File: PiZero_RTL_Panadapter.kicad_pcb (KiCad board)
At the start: 4 copper layers, 65 x 30 mm, 196 parts, among them J1 Conn_01x02, J2 JST GH 8 Position, J3 U.FL, J4 U.FL, J5 Conn_01x08, Q1 S8050T, Q2 BFS17, Q3 J310, Q4 BFS17, T1 DXW21BN2511NL, U1 RPM5.0-2.0, U10 SI5351B-B-GM1, U2 AP2114HA-3.3, U4 Raspberry Pi Zero 2W, U5 RTL2832U, U6 M24C02-WMN, U7 FE1.1s, U8 RTL8152B, U9 R820T2, Y1 25MHz

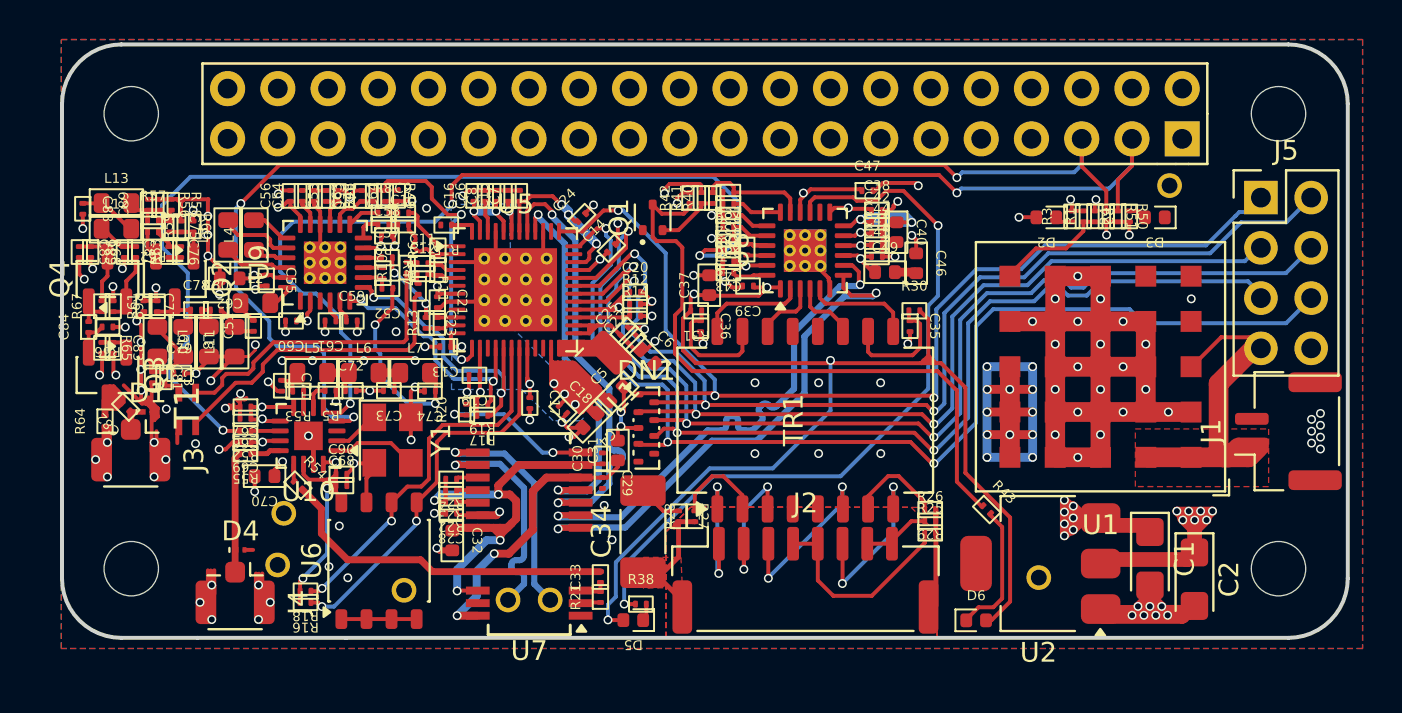
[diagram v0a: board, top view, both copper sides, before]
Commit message: PCB Layout finished?
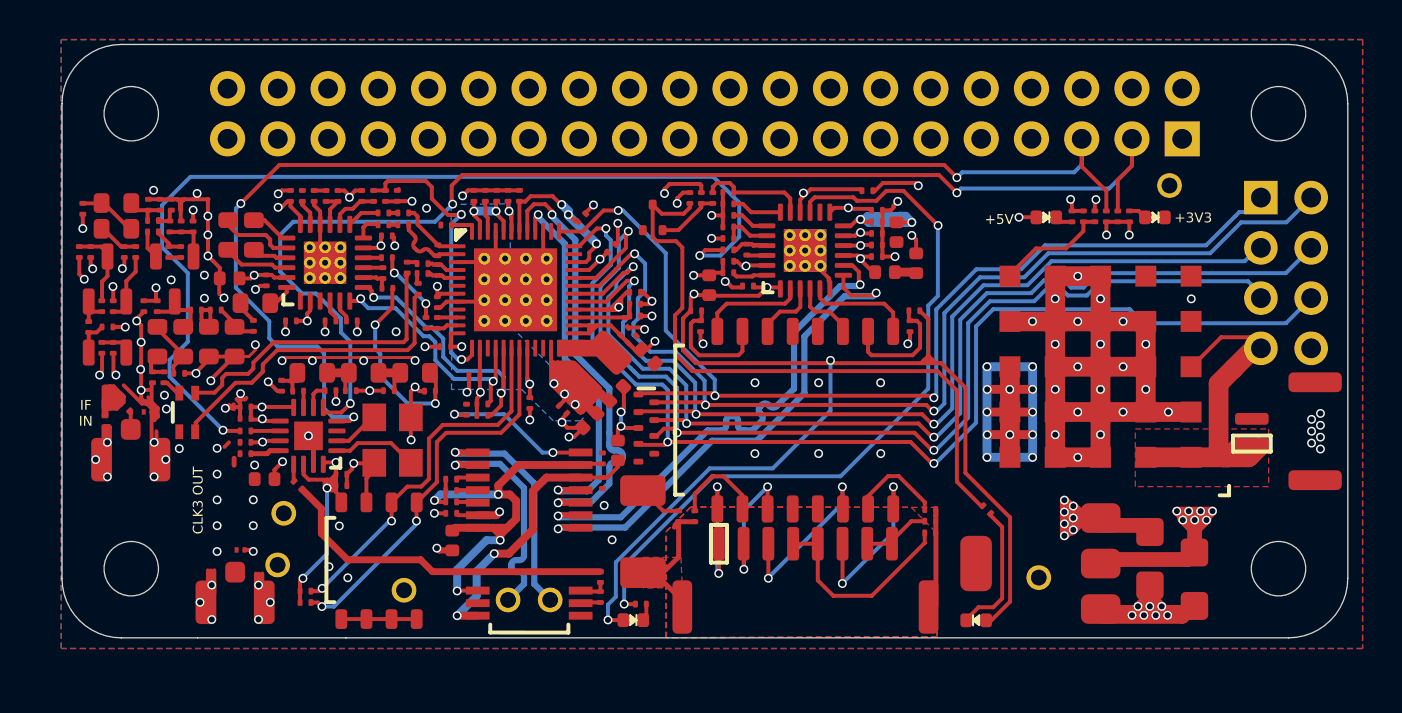
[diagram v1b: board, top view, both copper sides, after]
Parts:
- T1: footprint libraries:DXW21BN2511NL -> libraries:XFMR_ATB2012-50011-T000
- moved T1 0.15 mm to (124.8, 103.0), turned to 90 degrees
- moved C70 0.15 mm to (128.7, 106.3)
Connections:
- T1 pad 1: Net-(C3-Pad2) -> GND
- T1 pad 2: GND -> Net-(C3-Pad2)
- T1 pad 3: /IF_Q- -> /IF_Q+
- T1 pad 4: /IF_Q+ -> /IF_Q-
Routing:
- net GND: track 341.3 -> 354.6 mm, vias 125 -> 138
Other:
- board text added: "+3V3"
- board text added: "+5V"
- board text added: "CLK3 OUT"
- board text added: "IF IN"
